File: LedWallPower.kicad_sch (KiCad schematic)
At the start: 15 parts, among them U1 TPS5430DDA

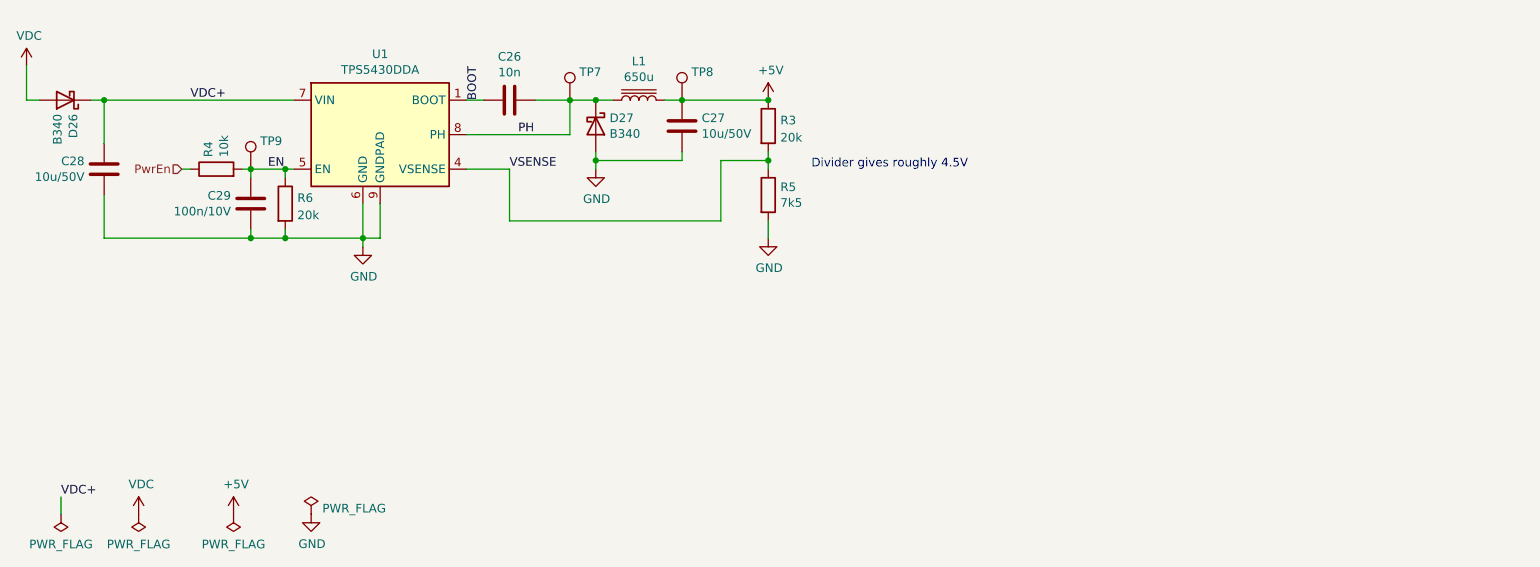
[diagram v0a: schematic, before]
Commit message: Change DC/DC components and split schematic
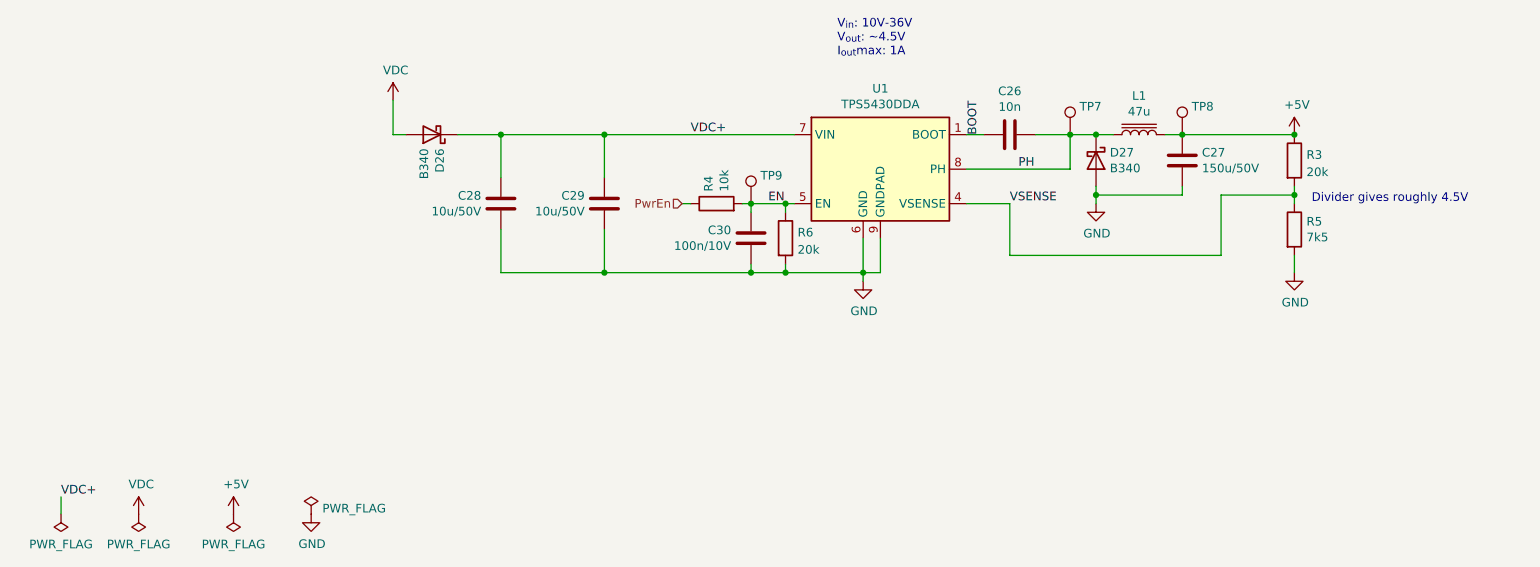
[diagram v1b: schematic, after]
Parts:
- added C28: 10u/50V, Capacitor_SMD:C_1206_3216Metric_Pad1.33x1.80mm_HandSolder, symbol Device:C
- C27: value 10u/50V -> 150u/50V; footprint Capacitor_SMD:C_1206_3216Metric_Pad1.33x1.80mm_HandSolder -> Capacitor_SMD:C_Elec_10x10.2; LCSC C13585 -> C72490
- L1: value 650u -> 47u; footprint Inductor_SMD:L_Bourns_SRR1208_12.7x12.7mm -> (none); LCSC C280641 -> C497841
- renumbered C28 to C29, C29 to C30
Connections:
- net GND: now also C28.1
- net VDC+: now also C28.2
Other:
- note added: "V_{in}: 10V-36V V_{out}: ~4.5V I_{out}max: 1A"
- moved on the sheet: C26, C27, C29, C30, D26, D27, L1, R3, R4, R5, R6, TP7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

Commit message: Change LED to one in JLC stock
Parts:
- L1: footprint (none) -> Ledwall:YNR6045-470M
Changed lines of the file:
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@@
     (property "Reference" "L1" (id 0) (at 193.04 47.625 90))
     (property "Value" "47u" (id 1) (at 193.04 49.9364 90))
-    (property "Footprint" "" (id 2) (at 193.04 53.34 0)
+    (property "Footprint" "Ledwall:YNR6045-470M" (id 2) (at 193.04 53.34 0)
       (effects (font (size 1.27 1.27)) hide)
     )

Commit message: Fix incorrect LCSC number for R3 and R6
Solves issue #1
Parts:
- R3, R6: LCSC C25805 -> C4184
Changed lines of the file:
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@@
       (effects (font (size 1.27 1.27)) hide)
     )
-    (property "LCSC" "C25805" (id 4) (at 215.9 57.15 0)
+    (property "LCSC" "C4184" (id 4) (at 215.9 57.15 0)
       (effects (font (size 1.27 1.27)) hide)
     )
@@
       (effects (font (size 1.27 1.27)) hide)
     )
-    (property "LCSC" "C25805" (id 4) (at 140.97 68.58 0)
+    (property "LCSC" "C4184" (id 4) (at 140.97 68.58 0)
       (effects (font (size 1.27 1.27)) hide)
     )
